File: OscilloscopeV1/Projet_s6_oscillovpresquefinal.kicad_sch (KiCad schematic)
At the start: 33 parts, among them IC1 PGA849RGTR, J1 Conn_Coaxial, J2 Conn_01x06_Socket, J3 PILES_3AA, J4 Conn_01x05_Pin, SW1 SW_SPST, U1 LM1117MP-5.0, U3 AP2112K-3.3, U4 STM32L476RGTx

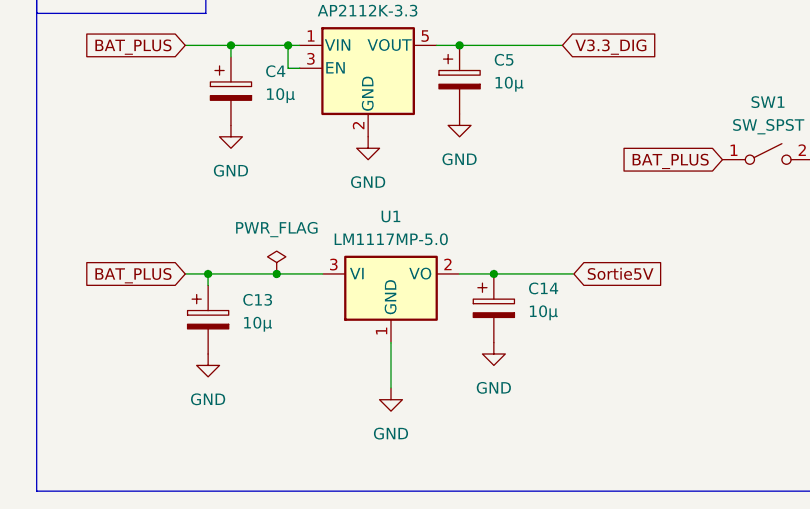
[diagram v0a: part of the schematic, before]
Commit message: Avancement PCB
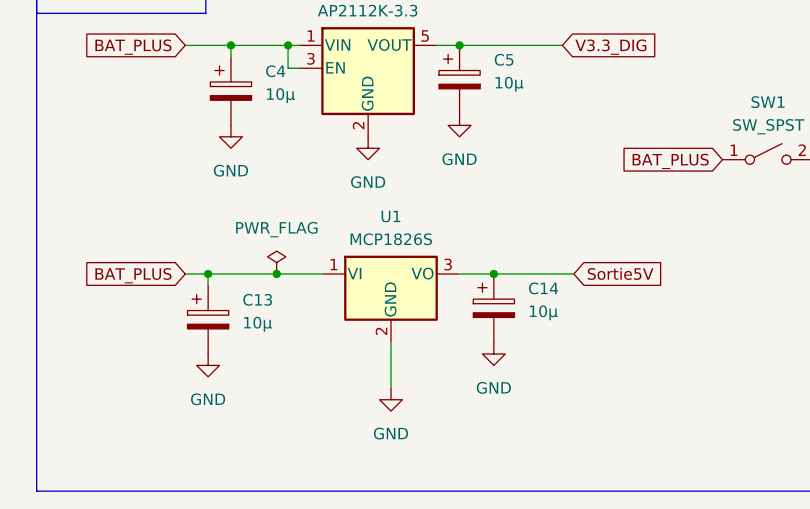
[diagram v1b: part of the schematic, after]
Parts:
- removed U1: LM1117MP-5.0, Package_TO_SOT_SMD:SOT-223-3_TabPin2, symbol Regulator_Linear:LM1117MP-5.0
- added U1: MCP1826S, Package_TO_SOT_SMD:SOT-223, symbol Regulator_Linear:MCP1826S
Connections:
- net BAT_PLUS: now also U1.1 (VI)
- net GND: now also U1.2 (GND)
- net Sortie5V: now also U1.3 (VO)
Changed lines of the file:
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@@
 	)
 	(junction
+		(at 199.39 231.14)
+		(diameter 0)
+		(color 0 0 0 0)
+	)
+	(junction
 		(at 292.1 224.79)
 		(diameter 0)
@@
 	)
 	(junction
+		(at 175.26 231.14)
+		(diameter 0)
+		(color 0 0 0 0)
+	)
+	(junction
 		(at 341.63 63.5)
 		(diameter 0)
@@
 	)
 	(junction
-		(at 175.26 231.14)
-		(diameter 0)
-		(color 0 0 0 0)
-	)
-	(junction
 		(at 167.64 231.14)
 		(diameter 0)
@@
 	)
 	(junction
-		(at 199.39 231.14)
-		(diameter 0)
-		(color 0 0 0 0)
-	)
-	(junction
 		(at 346.71 62.23)
 		(diameter 0)
@@
 	(wire
 		(pts
+			(xy 187.96 238.76) (xy 187.96 243.84)
+		)
+		(stroke
+			(width 0)
+			(type default)
+		)
+	)
+	(wire
+		(pts
 			(xy 74.93 135.89) (xy 80.01 135.89)
 		)
@@
 	(wire
 		(pts
+			(xy 175.26 231.14) (xy 180.34 231.14)
+		)
+		(stroke
+			(width 0)
+			(type default)
+		)
+	)
+	(wire
+		(pts
 			(xy 74.93 53.34) (xy 83.82 53.34)
 		)
@@
 	(wire
 		(pts
-			(xy 187.96 238.76) (xy 187.96 243.84)
-		)
-		(stroke
-			(width 0)
-			(type default)
-		)
-	)
-	(wire
-		(pts
 			(xy 292.1 229.87) (xy 292.1 233.68)
 		)
@@
 	(wire
 		(pts
-			(xy 199.39 231.14) (xy 195.58 231.14)
-		)
-		(stroke
-			(width 0)
-			(type default)
-		)
-	)
-	(wire
-		(pts
 			(xy 292.1 219.71) (xy 292.1 213.36)
 		)
@@
 	(wire
 		(pts
-			(xy 175.26 231.14) (xy 180.34 231.14)
-		)
-		(stroke
-			(width 0)
-			(type default)
-		)
-	)
-	(wire
-		(pts
 			(xy 60.96 241.3) (xy 72.39 241.3)
 		)
@@
 	(wire
 		(pts
+			(xy 195.58 231.14) (xy 199.39 231.14)
+		)
+		(stroke
+			(width 0)
+			(type default)
+		)
+	)
+	(wire
+		(pts
 			(xy 297.18 229.87) (xy 292.1 229.87)
 		)
@@
 	)
 	(symbol
+		(lib_id "Regulator_Linear:MCP1826S")
+		(at 187.96 231.14 0)
+		(unit 1)
+		(exclude_from_sim no)
+		(in_bom yes)
+		(on_board yes)
+		(dnp no)
+		(fields_autoplaced yes)
+		(property "Reference" "U1"
+			(at 187.96 224.79 0)
+			(effects
+				(font
+					(size 1.27 1.27)
+				)
+			)
+		)
+		(property "Value" "MCP1826S"
+			(at 187.96 227.33 0)
+			(effects
+				(font
+					(size 1.27 1.27)
+				)
+			)
+		)
+		(property "Footprint" "Package_TO_SOT_SMD:SOT-223"
+			(at 185.42 227.33 0)
+			(effects
+				(font
+					(size 1.27 1.27)
+				)
+				(hide yes)
+			)
+		)
+		(property "Datasheet" "http://ww1.microchip.com/downloads/en/DeviceDoc/22057B.pdf"
+			(at 187.96 224.79 0)
+			(effects
+				(font
+					(size 1.27 1.27)
+				)
+				(hide yes)
+			)
+		)
+		(property "Description" "1000mA, Low-Voltage, Low Quiescent Current LDO Regulator, SOT-223, TO-220, TO-263"
+			(at 187.96 231.14 0)
+			(effects
+				(font
+					(size 1.27 1.27)
+				)
+				(hide yes)
+			)
+		)
+		(pin "1"
+		)
+		(pin "2"
+		)
+		(pin "3"
+		)
+		(instances
+			(project ""
+				(path "/79a95597-2db4-4373-9cc6-70296586f172"
+					(reference "U1")
+					(unit 1)
+				)
+			)
+		)
+	)
+	(symbol
 		(lib_id "Device:C_Polarized")
 		(at 199.39 234.95 0)
@@
 					(unit 1)
 				)
-			)
-		)
-	)
-	(symbol
-		(lib_id "Regulator_Linear:LM1117MP-5.0")
-		(at 187.96 231.14 0)
-		(unit 1)
-		(exclude_from_sim no)
-		(in_bom yes)
-		(on_board yes)
-		(dnp no)
-		(fields_autoplaced yes)
-		(property "Reference" "U1"
-			(at 187.96 224.79 0)
-			(effects
-				(font
-					(size 1.27 1.27)
-				)
-			)
-		)
-		(property "Value" "LM1117MP-5.0"
-			(at 187.96 227.33 0)
-			(effects
-				(font
-					(size 1.27 1.27)
-				)
-			)
-		)
-		(property "Footprint" "Package_TO_SOT_SMD:SOT-223-3_TabPin2"
-			(at 187.96 231.14 0)
-			(effects
-				(font
-					(size 1.27 1.27)
-				)
-				(hide yes)
-			)
-		)
-		(property "Datasheet" "http://www.ti.com/lit/ds/symlink/lm1117.pdf"
-			(at 187.96 231.14 0)
-			(effects
-				(font
-					(size 1.27 1.27)
-				)
-				(hide yes)
-			)
-		)
-		(property "Description" "800mA Low-Dropout Linear Regulator, 5.0V fixed output, SOT-223"
-			(at 187.96 231.14 0)
-			(effects
-				(font
-					(size 1.27 1.27)
-				)
-				(hide yes)
-			)
-		)
-		(pin "3"
-		)
-		(pin "1"
-		)
-		(pin "2"
-		)
-		(instances
-			(project ""
-				(path "/79a95597-2db4-4373-9cc6-70296586f172"
-					(reference "U1")
-					(unit 1)
-				)
